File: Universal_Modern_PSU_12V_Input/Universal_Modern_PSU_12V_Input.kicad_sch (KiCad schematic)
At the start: 24 parts, among them J1 +12VDC Input, J2 Power Output, Q1 SUP53P06-20-E3, U1 DFR0831, U2 NKE1212SC, U3 R-78CK5.0-0.5

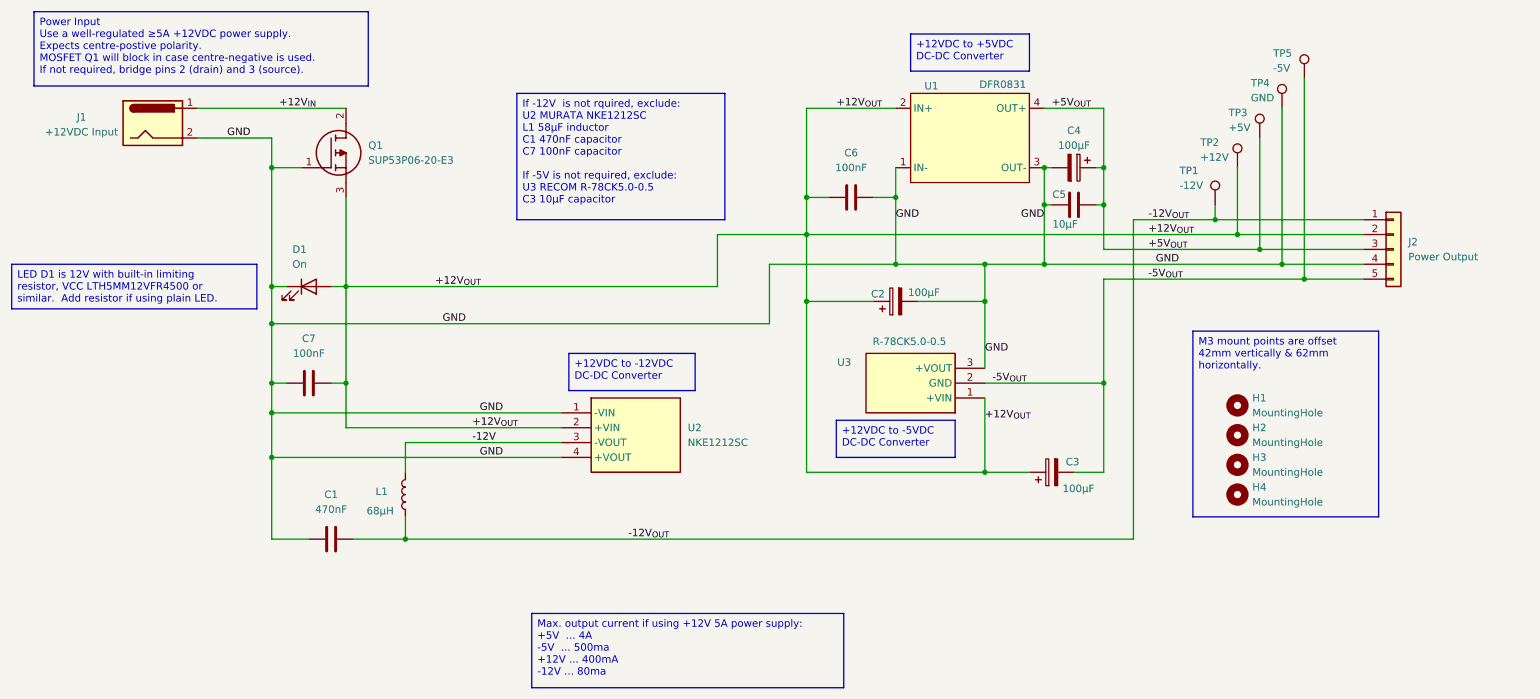
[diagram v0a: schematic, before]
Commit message: Minor PCB & schematic changes
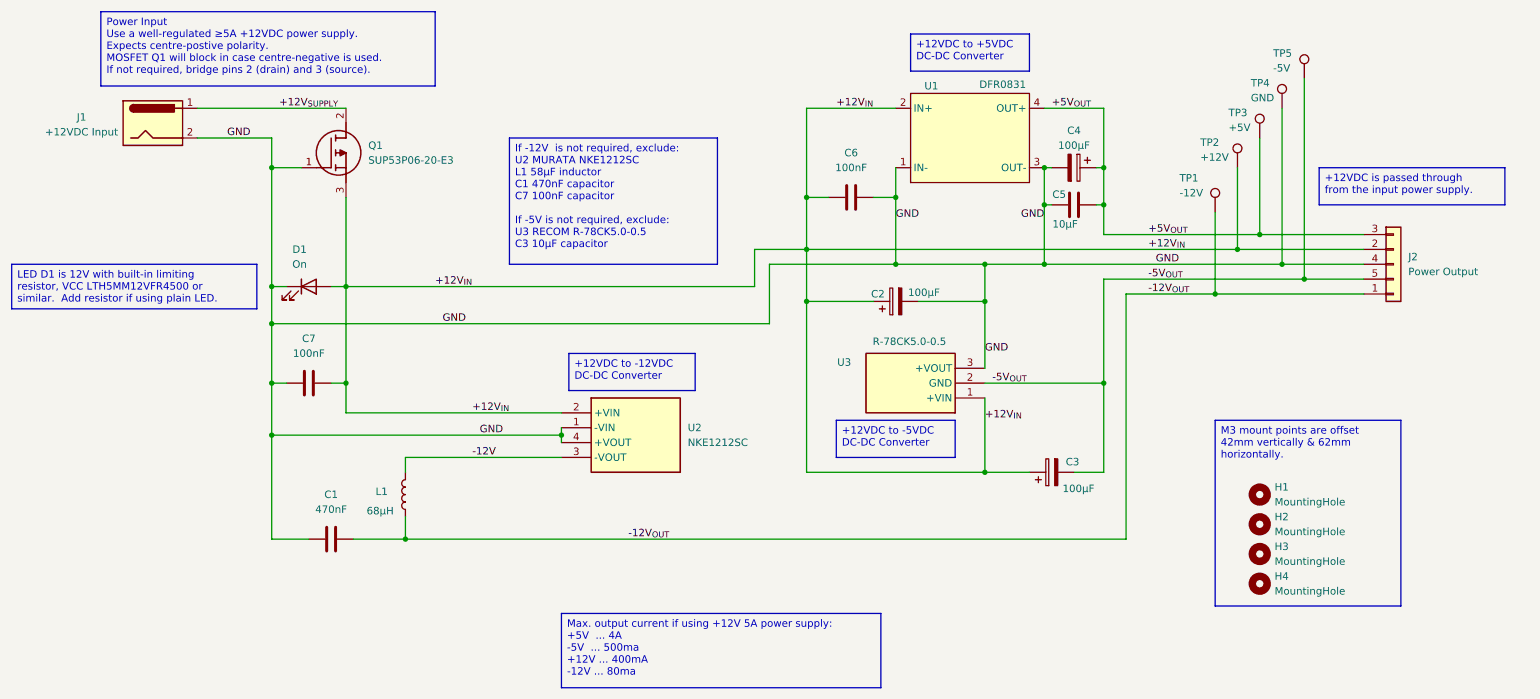
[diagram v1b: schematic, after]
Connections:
- net +12V_{OUT} is gone; now on net +12V_{IN}: C2.1, C3.1, C6.1, C7.2, D1.2 (A), J2.2 (Pin_2), Q1.3 (S), TP2.1, U1.2 (IN+), U2.2 (+VIN), U3.1 (+VIN)
- net +12V_{IN}: no longer J1.1, Q1.2 (D)
- new net +12V_{SUPPLY}: J1.1, Q1.2 (D)
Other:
- moved on the sheet: H1, H2, H3, H4, J2, TP1
